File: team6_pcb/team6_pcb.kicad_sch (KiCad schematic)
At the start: 26 parts, among them P10 MAB, P2 STEP/DIR, P3 MISC, P4 Conn_01x01, P5 Conn_01x01, P8 VCC_IO, P9 VM, Q1 SI4532CDY-T1-GE3, Q2 SI4532CDY-T1-GE3, Q3 SI4532CDY-T1-GE3, Q4 SI4532CDY-T1-GE3

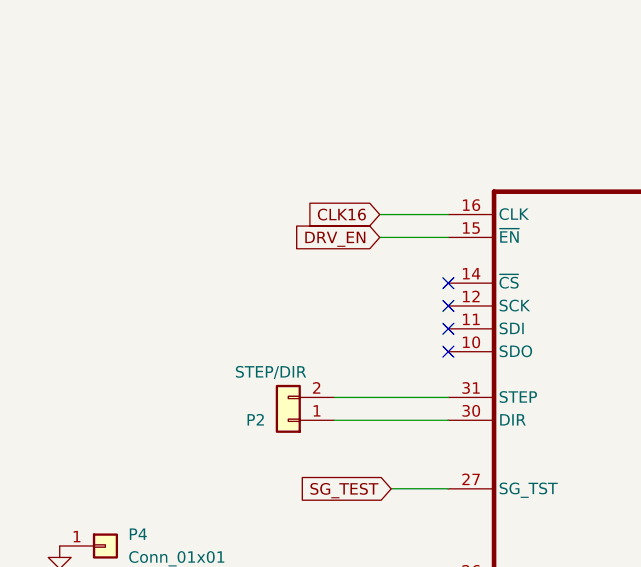
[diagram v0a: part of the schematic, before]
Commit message: team6_final_sumbits
Adin Stamped
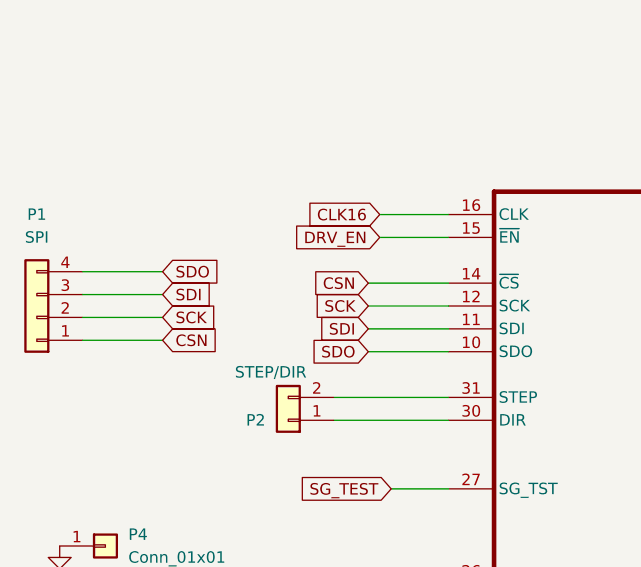
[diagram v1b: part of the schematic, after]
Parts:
- added P1: SPI, Connector_PinHeader_2.54mm:PinHeader_1x04_P2.54mm_Vertical, symbol Connector_Generic:Conn_01x04
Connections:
- net SDO: now reaches IC1.10 (SDO)
- net SDO: now also P1.4 (Pin_4)
- net SDI: now reaches IC1.11 (SDI)
- net SDI: now also P1.3 (Pin_3)
- net SCK: now reaches IC1.12 (SCK)
- net SCK: now also P1.2 (Pin_2)
- net CSN: now reaches IC1.14 (~{CS})
- net CSN: now also P1.1 (Pin_1)
- no-connect marks 5 -> 1
